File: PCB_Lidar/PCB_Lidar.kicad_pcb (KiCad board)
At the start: 2 copper layers, 54 x 45.8 mm, 47 parts, among them J1 5VP, J2 CON_CAN, J3 USB_C_Receptacle_USB2.0, J4 CON_LIDAR, J5 CON_CAN, U1 SN65HVD232, U2 NCP1117-3.3_SOT223, U3 STM32F302C6Tx, Y1 8MHz

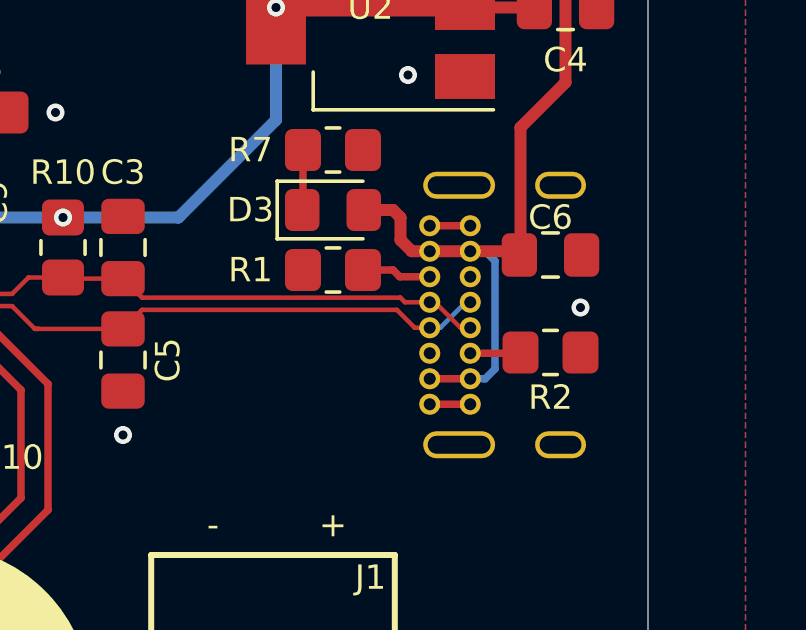
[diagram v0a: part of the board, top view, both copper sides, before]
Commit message: Beaucoup de chose
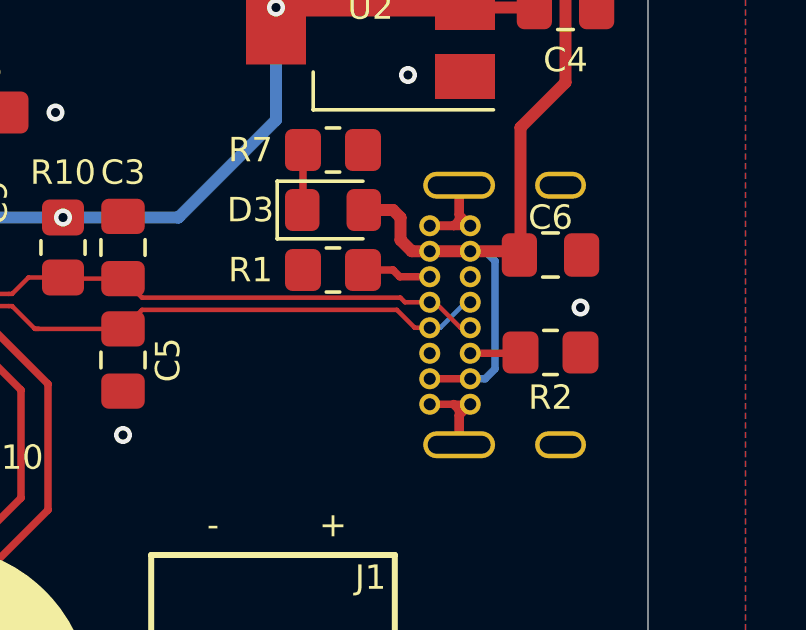
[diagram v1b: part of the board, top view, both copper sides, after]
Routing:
- net GND: track 12.2 -> 19.4 mm
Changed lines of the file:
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@@
   (segment (start 201.075 92.375) (end 200.575 92.375) (width 0.25) (layer "B.Cu") (net 1))
   (segment (start 201.4 92.7) (end 201.075 92.375) (width 0.25) (layer "B.Cu") (net 1))
+  (segment (start 200.025 91.525) (end 200.205 91.345) (width 0.3) (layer "F.Cu") (net 2))
+  (segment (start 200.205 97.655) (end 200.205 98.825) (width 0.3) (layer "F.Cu") (net 2))
   (segment (start 174.25 89.5) (end 174.25 90.8375) (width 0.25) (layer "F.Cu") (net 2))
   (segment (start 199.25 91.5) (end 199.275 91.525) (width 0.25) (layer "F.Cu") (net 2))
+  (segment (start 200.575 97.475) (end 200.205 97.845) (width 0.3) (layer "F.Cu") (net 2))
+  (segment (start 200.205 91.155) (end 200.575 91.525) (width 0.3) (layer "F.Cu") (net 2))
   (segment (start 178.75 97.5) (end 178.75 99.1625) (width 0.3) (layer "F.Cu") (net 2))
-  (segment (start 199.225 97.475) (end 200.575 97.475) (width 0.25) (layer "F.Cu") (net 2))
+  (segment (start 200.205 97.845) (end 200.205 98.825) (width 0.3) (layer "F.Cu") (net 2))
+  (segment (start 200.025 97.475) (end 200.205 97.655) (width 0.3) (layer "F.Cu") (net 2))
+  (segment (start 200.025 97.475) (end 200.575 97.475) (width 0.25) (layer "F.Cu") (net 2))
+  (segment (start 199.225 97.475) (end 200.025 97.475) (width 0.25) (layer "F.Cu") (net 2))
+  (segment (start 200.025 91.525) (end 199.225 91.525) (width 0.3) (layer "F.Cu") (net 2))
   (segment (start 172.725 82.385) (end 175.0975 82.385) (width 0.3) (layer "F.Cu") (net 2))
   (segment (start 175.0975 82.385) (end 175.5 82.7875) (width 0.3) (layer "F.Cu") (net 2))
+  (segment (start 200.205 90.175) (end 200.205 91.155) (width 0.3) (layer "F.Cu") (net 2))
   (segment (start 180.6625 92.75) (end 182.5 92.75) (width 0.25) (layer "F.Cu") (net 2))
+  (segment (start 200.205 91.345) (end 200.205 90.175) (width 0.3) (layer "F.Cu") (net 2))
   (segment (start 199.275 91.525) (end 200.575 91.525) (width 0.25) (layer "F.Cu") (net 2))
+  (segment (start 200.575 91.525) (end 200.025 91.525) (width 0.3) (layer "F.Cu") (net 2))
   (segment (start 172.3375 95.75) (end 173.75 95.75) (width 0.3) (layer "F.Cu") (net 2))
   (segment (start 174 89.25) (end 174.25 89.5) (width 0.25) (layer "F.Cu") (net 2))
